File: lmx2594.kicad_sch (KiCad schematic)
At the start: 46 parts, among them J36 SYSREFREQ, J37 TUNESENSE, U22 LMX2594

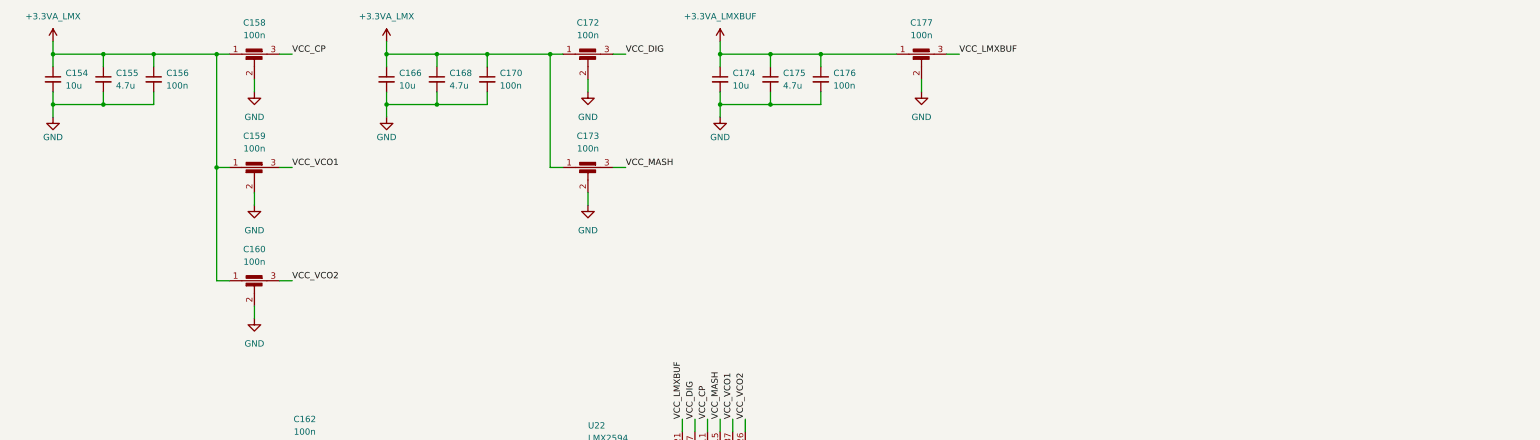
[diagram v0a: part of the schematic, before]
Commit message: wip
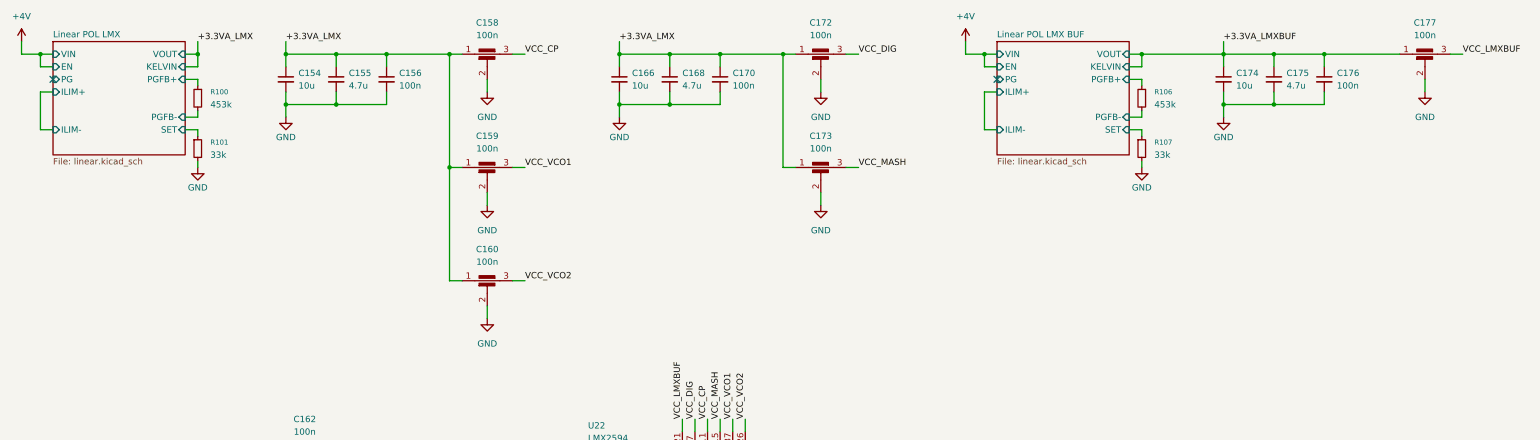
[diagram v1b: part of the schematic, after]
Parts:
- added R100, R106: 453k, Resistor_SMD:R_0402_1005Metric, symbol Device:R_Small
- added R101, R107: 33k, Resistor_SMD:R_0402_1005Metric, symbol Device:R_Small
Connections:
- net GND: now also R101.2, R107.2
- new net Linear POL LMX BUF/PGFB+: R106.1
- new net Linear POL LMX BUF/PGFB-: R106.2
- new net Linear POL LMX BUF/SET: R107.1
- new net Linear POL LMX/PGFB+: R100.1
- new net Linear POL LMX/PGFB-: R100.2
- new net Linear POL LMX/SET: R101.1
- no-connect marks 0 -> 2
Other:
- added sheet Linear POL LMX (linear.kicad_sch)
- added sheet Linear POL LMX BUF (linear.kicad_sch)
- moved on the sheet: C154, C155, C156, C158, C159, C160, C166, C168, C170, C172, C173, C174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
